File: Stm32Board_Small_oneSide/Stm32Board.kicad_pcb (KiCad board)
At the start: 2 copper layers, 30.4 x 25.2 mm, 58 parts, among them J1 USB_B_Micro, SW1 SW_Push, U1 STM32L151CBTx, U2 XC6210B332MR, Y1 32k, Y2 12Mhz

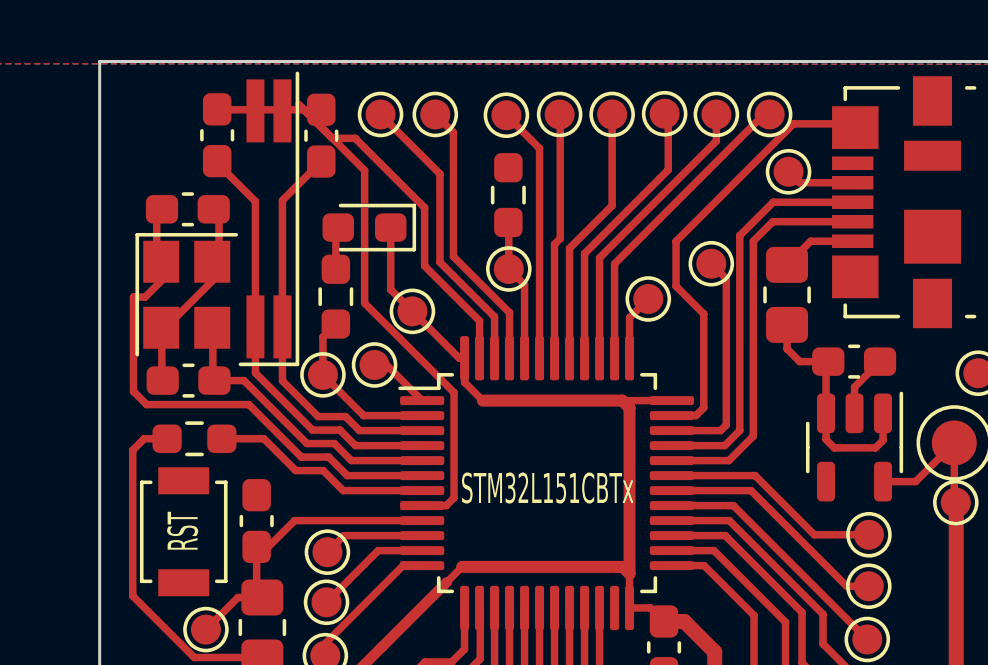
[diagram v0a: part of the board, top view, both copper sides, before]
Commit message: Added GRB
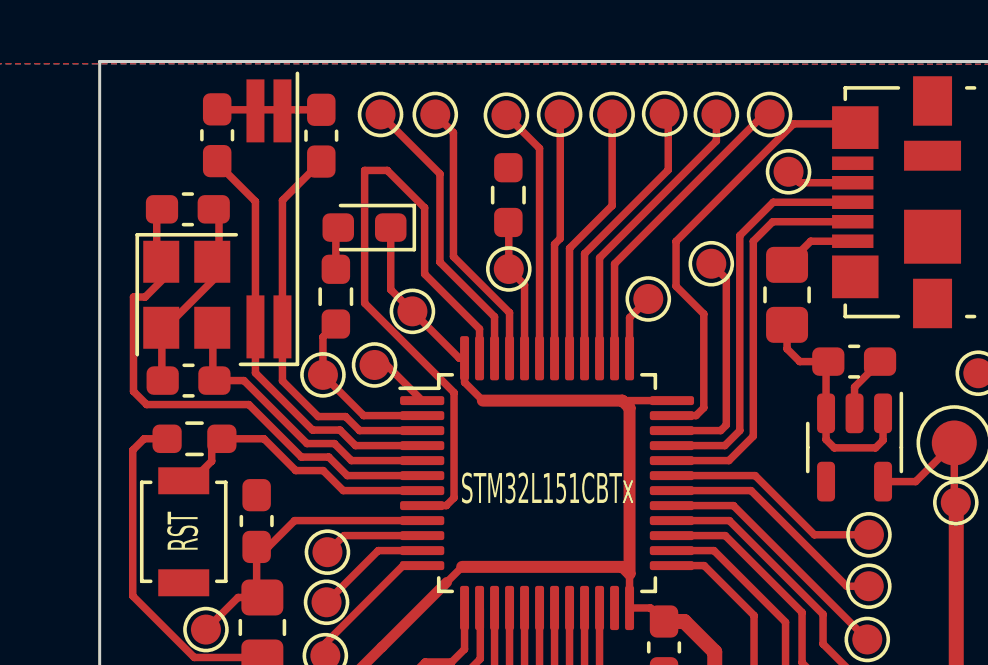
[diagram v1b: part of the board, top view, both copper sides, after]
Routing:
- net GND: track 53.8 -> 47.6 mm
- net Net-(U1-NRST): track 7.39 -> 9.48 mm
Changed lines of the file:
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@@
     (grid_origin 119.634 0)
     (pcbplotparams
-      (layerselection 0x0001020_ffffffff)
+      (layerselection 0x00010a0_7fffffff)
       (plot_on_all_layers_selection 0x0000000_00000000)
       (disableapertmacros false)
@@
     (fp_line (start 1 0.625) (end -1 0.625)
       (stroke (width 0.1) (type solid)) (layer "F.Fab"))
-    (pad "1" smd roundrect (at -1 0 270) (size 1.2 1.4) (layers "F.Cu" "F.Paste" "F.Mask") (roundrect_rratio 0.208333)
+    (pad "1" smd roundrect (at -1 0 270) (size 1.2 1.4) (layers "F.Cu" "F.Paste" "F.Mask") (roundrect_rratio 0.2083333333)
       (net 8 "+5V") (pintype "passive"))
-    (pad "2" smd roundrect (at 1 0 270) (size 1.2 1.4) (layers "F.Cu" "F.Paste" "F.Mask") (roundrect_rratio 0.208333)
+    (pad "2" smd roundrect (at 1 0 270) (size 1.2 1.4) (layers "F.Cu" "F.Paste" "F.Mask") (roundrect_rratio 0.2083333333)
       (net 6 "Net-(U2-CE)") (pintype "passive"))
     (model "${KICAD6_3DMODEL_DIR}/Resistor_SMD.3dshapes/R_0805_2012Metric.wrl"
@@
       (net 11 "Net-(U1-NRST)") (pinfunction "NRST") (pintype "input"))
     (pad "8" smd roundrect (at -4.1625 0.75) (size 1.475 0.3) (layers "F.Cu" "F.Paste" "F.Mask") (roundrect_rratio 0.25)
-      (net 2 "GND") (pinfunction "VSSA") (pintype "power_in"))
+      (net 2 "GND") (pinfunction "VSSA") (pintype "power_in") (zone_connect 2))
     (pad "9" smd roundrect (at -4.1625 1.25) (size 1.475 0.3) (layers "F.Cu" "F.Paste" "F.Mask") (roundrect_rratio 0.25)
       (net 9 "Net-(U1-VDDA)") (pinfunction "VDDA") (pintype "power_in"))
@@
       (net 25 "Net-(U1-PB11)") (pinfunction "PB11") (pintype "bidirectional"))
     (pad "23" smd roundrect (at 2.25 4.1625) (size 0.3 1.475) (layers "F.Cu" "F.Paste" "F.Mask") (roundrect_rratio 0.25)
-      (net 2 "GND") (pinfunction "VSS") (pintype "power_in"))
+      (net 2 "GND") (pinfunction "VSS") (pintype "power_in") (zone_connect 2))
     (pad "24" smd roundrect (at 2.75 4.1625) (size 0.3 1.475) (layers "F.Cu" "F.Paste" "F.Mask") (roundrect_rratio 0.25)
       (net 7 "+3.3V") (pinfunction "VDD") (pintype "power_in"))
@@
       (net 32 "Net-(U1-PA13)") (pinfunction "PA13") (pintype "bidirectional"))
     (pad "35" smd roundrect (at 4.1625 -2.25) (size 1.475 0.3) (layers "F.Cu" "F.Paste" "F.Mask") (roundrect_rratio 0.25)
-      (net 2 "GND") (pinfunction "VSS") (pintype "passive"))
+      (net 2 "GND") (pinfunction "VSS") (pintype "passive") (zone_connect 2))
     (pad "36" smd roundrect (at 4.1625 -2.75) (size 1.475 0.3) (layers "F.Cu" "F.Paste" "F.Mask") (roundrect_rratio 0.25)
       (net 7 "+3.3V") (pinfunction "VDD") (pintype "power_in"))
@@
       (net 23 "Net-(U1-PB9)") (pinfunction "PB9") (pintype "bidirectional"))
     (pad "47" smd roundrect (at -2.25 -4.1625) (size 0.3 1.475) (layers "F.Cu" "F.Paste" "F.Mask") (roundrect_rratio 0.25)
-      (net 2 "GND") (pinfunction "VSS") (pintype "passive"))
+      (net 2 "GND") (pinfunction "VSS") (pintype "passive") (zone_connect 2))
     (pad "48" smd roundrect (at -2.75 -4.1625) (size 0.3 1.475) (layers "F.Cu" "F.Paste" "F.Mask") (roundrect_rratio 0.25)
       (net 7 "+3.3V") (pinfunction "VDD") (pintype "power_in"))
@@
   (segment (start 159.131208 85.52) (end 160.044812 85.52) (width 0.25) (layer "F.Cu") (net 1))
   (segment (start 156.0465 83.42) (end 157.031208 83.42) (width 0.25) (layer "F.Cu") (net 1))
-  (segment (start 164.034 83.82) (end 164.034 87.328185) (width 0.25) (layer "F.Cu") (net 2))
-  (segment (start 158.854 74.215) (end 161.054 76.415) (width 0.25) (layer "F.Cu") (net 2))
-  (segment (start 163.774685 87.5875) (end 162.9715 87.5875) (width 0.25) (layer "F.Cu") (net 2))
+  (segment (start 164.034 87.328185) (end 163.774685 87.5875) (width 0.25) (layer "F.Cu") (net 2))
   (segment (start 155.994 80.08) (end 154.294 81.78) (width 0.25) (layer "F.Cu") (net 2))
-  (segment (start 164.884 82.675) (end 164.884 81.430787) (width 0.25) (layer "F.Cu") (net 2))
   (segment (start 159.609 74.394) (end 156.184 74.394) (width 0.25) (layer "F.Cu") (net 2))
+  (segment (start 163.054 77.66) (end 161.809 76.415) (width 0.25) (layer "F.Cu") (net 2))
   (segment (start 172.359 81.2) (end 171.434 80.275) (width 0.25) (layer "F.Cu") (net 2))
   (segment (start 171.434 78.78) (end 175.3515 74.8625) (width 0.25) (layer "F.Cu") (net 2))
   (segment (start 171.2965 84.5875) (end 172.099685 84.5875) (width 0.25) (layer "F.Cu") (net 2))
-  (segment (start 160.739 75.345) (end 159.984 75.345) (width 0.25) (layer "F.Cu") (net 2))
+  (segment (start 163.774685 87.5875) (end 162.9715 87.5875) (width 0.25) (layer "F.Cu") (net 2))
+  (segment (start 164.884 82.675) (end 164.884 81.699) (width 0.25) (layer "F.Cu") (net 2))
+  (segment (start 164.884 81.699) (end 163.054 79.869) (width 0.25) (layer "F.Cu") (net 2))
   (segment (start 171.434 80.275) (end 171.434 78.78) (width 0.25) (layer "F.Cu") (net 2))
   (segment (start 161.054 76.415) (end 161.054 80.84) (width 0.25) (layer "F.Cu") (net 2))
-  (segment (start 161.054 80.84) (end 164.034 83.82) (width 0.25) (layer "F.Cu") (net 2))
   (segment (start 177.384 83.6375) (end 177.384 84.5125) (width 0.25) (layer "F.Cu") (net 2))
   (segment (start 154.294 82.03) (end 154.294 83.3925) (width 0.25) (layer "F.Cu") (net 2))
   (segment (start 175.3515 74.8625) (end 177.284 74.8625) (width 0.25) (layer "F.Cu") (net 2))
   (segment (start 154.294 83.3925) (end 154.3215 83.42) (width 0.25) (layer "F.Cu") (net 2))
-  (segment (start 164.884 81.430787) (end 163.054 79.600787) (width 0.25) (layer "F.Cu") (net 2))
-  (segment (start 164.034 87.328185) (end 163.774685 87.5875) (width 0.25) (layer "F.Cu") (net 2))
-  (segment (start 159.984 75.345) (end 158.854 74.215) (width 0.25) (layer "F.Cu") (net 2))
+  (segment (start 164.034 83.82) (end 164.034 87.328185) (width 0.25) (layer "F.Cu") (net 2))
+  (segment (start 163.054 79.869) (end 163.054 77.66) (width 0.25) (layer "F.Cu") (net 2))
+  (segment (start 161.054 80.84) (end 164.034 83.82) (width 0.25) (layer "F.Cu") (net 2))
   (segment (start 172.359 84.328185) (end 172.359 81.2) (width 0.25) (layer "F.Cu") (net 2))
   (segment (start 177.284 74.8625) (end 177.409 74.9875) (width 0.25) (layer "F.Cu") (net 2))
-  (segment (start 163.054 79.600787) (end 163.054 77.66) (width 0.25) (layer "F.Cu") (net 2))
   (segment (start 156.199 77.712) (end 156.199 79.625) (width 0.25) (layer "F.Cu") (net 2))
   (segment (start 178.234 82.7875) (end 177.384 83.6375) (width 0.25) (layer "F.Cu") (net 2))
-  (segment (start 163.054 77.66) (end 160.739 75.345) (width 0.25) (layer "F.Cu") (net 2))
   (segment (start 172.099685 84.5875) (end 172.359 84.328185) (width 0.25) (layer "F.Cu") (net 2))
+  (segment (start 161.809 76.415) (end 161.054 76.415) (width 0.25) (layer "F.Cu") (net 2))
   (segment (start 153.739 80.635) (end 153.349 80.635) (width 0.25) (layer "F.Cu") (net 3))
   (segment (start 159.858416 85.97) (end 160.475916 86.5875) (width 0.25) (layer "F.Cu") (net 3))
@@
   (segment (start 166.384 82.675) (end 166.384 80.225) (width 0.25) (layer "F.Cu") (net 10))
   (segment (start 165.859 79.7) (end 165.859 78.165) (width 0.25) (layer "F.Cu") (net 10))
+  (segment (start 155.956 85.698) (end 156.294 85.36) (width 0.25) (layer "F.Cu") (net 11))
   (segment (start 158.758416 86.42) (end 157.698416 85.36) (width 0.25) (layer "F.Cu") (net 11))
   (segment (start 157.698416 85.36) (end 156.294 85.36) (width 0.25) (layer "F.Cu") (net 11))
+  (segment (start 155.956 86.106) (end 155.956 85.698) (width 0.25) (layer "F.Cu") (net 11))
   (segment (start 160.33952 87.0875) (end 159.67202 86.42) (width 0.25) (layer "F.Cu") (net 11))
   (segment (start 162.9715 87.0875) (end 160.33952 87.0875) (width 0.25) (layer "F.Cu") (net 11))
+  (segment (start 155.302 86.76) (end 155.956 86.106) (width 0.25) (layer "F.Cu") (net 11))
+  (segment (start 155.024 86.76) (end 155.302 86.76) (width 0.25) (layer "F.Cu") (net 11))
   (segment (start 159.67202 86.42) (end 158.758416 86.42) (width 0.25) (layer "F.Cu") (net 11))
   (segment (start 177.324 76.825) (end 175.549 76.825) (width 0.25) (layer "F.Cu") (net 12))
@@
       )
     )
+  )
+  (zone (net 0) (net_name "") (layer "F.Cu") (hatch edge 0.5)
+    (connect_pads (clearance 0))
+    (min_thickness 0.25) (filled_areas_thickness no)
+    (keepout (tracks allowed) (vias not_allowed) (pads not_allowed) (copperpour not_allowed) (footprints allowed))
+    (fill (thermal_gap 0.5) (thermal_bridge_width 0.5))
+    (polygon
+      (pts
+        (xy 178.816 75.946)
+        (xy 178.816 79.248)
+        (xy 178.054 79.248)
+        (xy 178.054 75.946)
+      )
+    )
